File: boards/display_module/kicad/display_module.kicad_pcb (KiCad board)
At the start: 2 copper layers, 58.4 x 148.6 mm, 35 parts, among them IC1 ATMEGA328-P, P1 CONN_01X02, Q1 NDP6020P, Q2 NDP6020P, Q3 NDP6020P, Q4 NDP6020P, Q5 NDP6020P, Q6 NDP6020P, Q7 NDP6020P, Q8 NDP6020P, U1 TLC5940NT, U2 TLC5940NT, Y1 16M

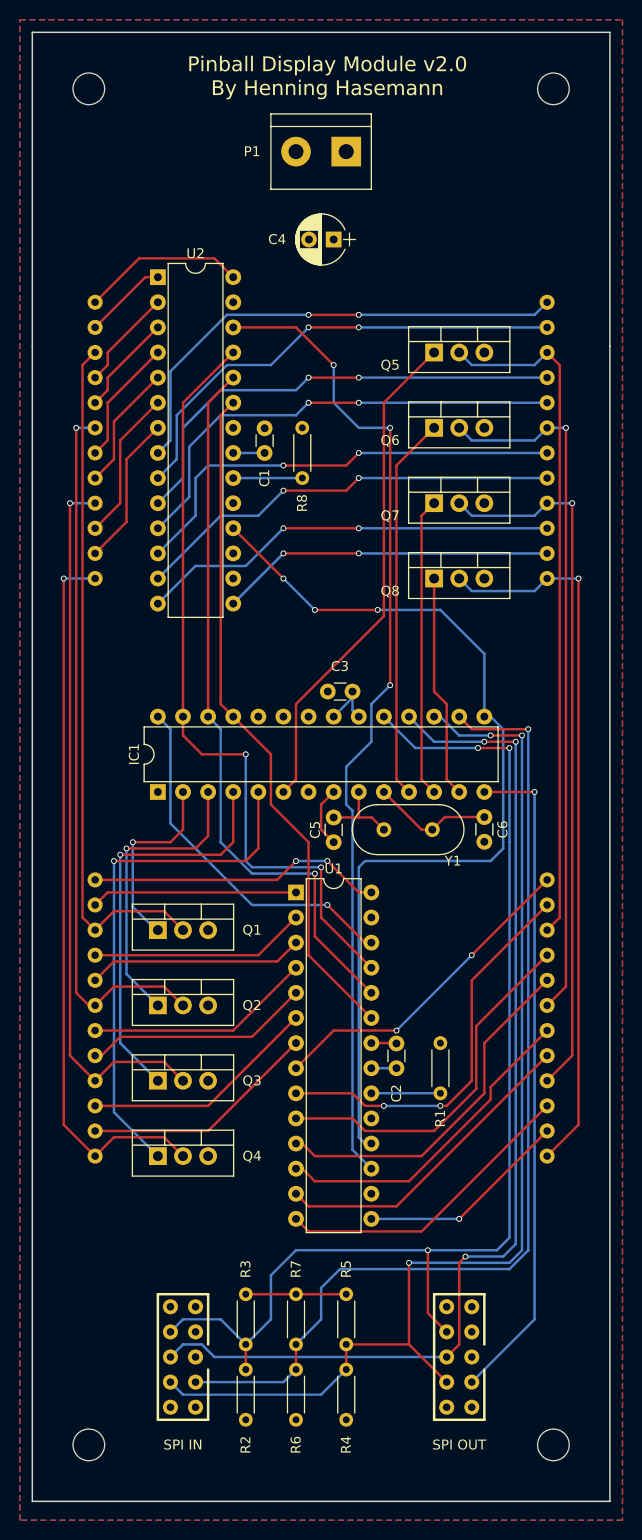
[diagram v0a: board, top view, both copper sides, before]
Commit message: WIP: display module PCB design v2.1
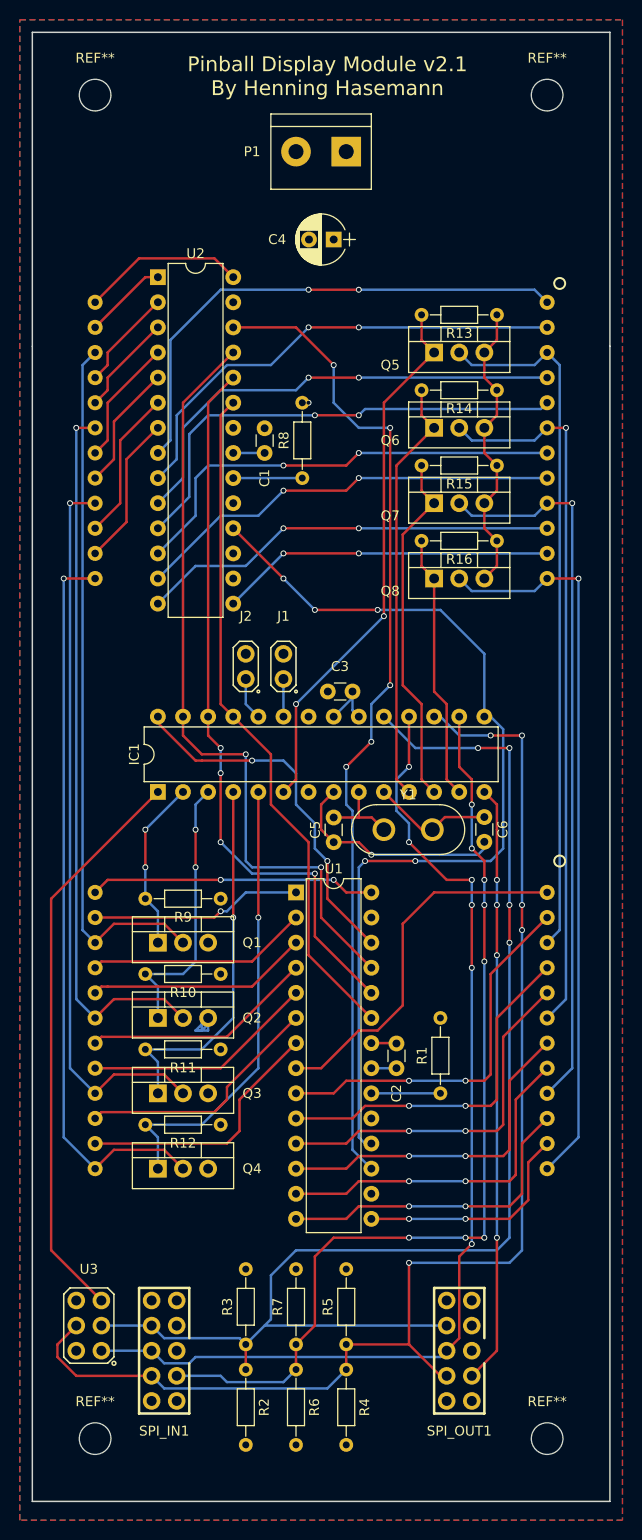
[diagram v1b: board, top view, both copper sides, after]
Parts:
- removed ? (x4): , Mounting_Holes:MountingHole_3.2mm_M3_DIN965
- removed SPI IN: SW10, my_footprints:SW10
- removed SPI OUT: SW10, my_footprints:SW10
- added J1: SELFTEST, my_footprints:PINS1x2, F.Cu at (144.8, 104.8)
- added J2: AUX, my_footprints:PINS1x2, F.Cu at (141.0, 104.8)
- added R10: 10k, Resistors_ThroughHole:R_Axial_DIN0204_L3.6mm_D1.6mm_P7.62mm_Horizontal, F.Cu at (138.4, 139.7)
- added R11: 10k, Resistors_ThroughHole:R_Axial_DIN0204_L3.6mm_D1.6mm_P7.62mm_Horizontal, F.Cu at (138.4, 147.3)
- added R12: 10k, Resistors_ThroughHole:R_Axial_DIN0204_L3.6mm_D1.6mm_P7.62mm_Horizontal, F.Cu at (138.4, 154.9)
- added R13: 10k, Resistors_ThroughHole:R_Axial_DIN0204_L3.6mm_D1.6mm_P7.62mm_Horizontal, F.Cu at (166.4, 73.0)
- added R14: 10k, Resistors_ThroughHole:R_Axial_DIN0204_L3.6mm_D1.6mm_P7.62mm_Horizontal, F.Cu at (166.4, 80.6)
- added R15: 10k, Resistors_ThroughHole:R_Axial_DIN0204_L3.6mm_D1.6mm_P7.62mm_Horizontal, F.Cu at (166.4, 88.3)
- added R16: 10k, Resistors_ThroughHole:R_Axial_DIN0204_L3.6mm_D1.6mm_P7.62mm_Horizontal, F.Cu at (166.4, 95.9)
- added R9: 10k, Resistors_ThroughHole:R_Axial_DIN0204_L3.6mm_D1.6mm_P7.62mm_Horizontal, F.Cu at (138.4, 132.1)
- added REF**: MountingHole_3.2mm_M3_ISO14580, Mounting_Holes:MountingHole_3.2mm_M3_ISO14580, F.Cu at (171.4, 50.8)
- added REF**: MountingHole_3.2mm_M3_ISO14580, Mounting_Holes:MountingHole_3.2mm_M3_ISO14580, F.Cu at (125.7, 50.8)
- added REF**: MountingHole_3.2mm_M3_ISO14580, Mounting_Holes:MountingHole_3.2mm_M3_ISO14580, F.Cu at (125.7, 186.7)
- added REF**: MountingHole_3.2mm_M3_ISO14580, Mounting_Holes:MountingHole_3.2mm_M3_ISO14580, F.Cu at (171.4, 186.7)
- added SPI_IN1: SW10, my_footprints:SW10, F.Cu at (132.7, 185.4)
- added SPI_OUT1: SW10, my_footprints:SW10, F.Cu at (162.6, 185.4)
- added U3: ICSP, my_footprints:PINS3x2, F.Cu at (125.1, 170.8)
- P1: value CONN_01X02 -> POWER
- R1, R2, R3, R4, R5, R6, R7, R8: footprint Resistors_ThroughHole:R_Axial_DIN0204_L3.6mm_D1.6mm_P5.08mm_Horizontal -> Resistors_ThroughHole:R_Axial_DIN0204_L3.6mm_D1.6mm_P7.62mm_Horizontal
- Y1: footprint Crystals:Crystal_HC18-U_Vertical -> Crystals:Crystal_HC50_Vertical
- moved Q1 1.27 mm to (132.1, 136.5)
- moved Q2 1.27 mm to (132.1, 144.1)
- moved DISP1 1.27 mm to (148.6, 141.6)
- moved Q3 1.27 mm to (132.1, 151.8)
- moved Q4 1.27 mm to (132.1, 159.4)
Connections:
- IC1 pad 1: (no net) -> Net-(IC1-Pad1)
- IC1 pad 23: (no net) -> Net-(IC1-Pad23)
- IC1 pad 24: (no net) -> Net-(IC1-Pad24)
- U1 pad 16: (no net) -> Net-(U1-Pad16)
- U2 pad 16: (no net) -> Net-(U2-Pad16)
- U2 pad 17: (no net) -> Net-(U2-Pad17)
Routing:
- net Net-(IC1-Pad1): track 0.00 -> 58.0 mm
- net VCC: track 22.0 -> 51.5 mm
- net GND: track 8.69 -> 25.4 mm, vias 0 -> 2
- net Net-(IC1-Pad17): track 115.6 -> 131.3 mm, vias 3 -> 5
- net Net-(IC1-Pad19): track 118.1 -> 133.6 mm, vias 3 -> 4
- net Net-(IC1-Pad14): track 67.4 -> 60.6 mm, vias 1 -> 4
- net Net-(IC1-Pad16): track 102.7 -> 96.8 mm, vias 1 -> 8
- net Net-(IC1-Pad12): track 30.3 -> 36.2 mm
- net Net-(IC1-Pad5): track 52.5 -> 46.7 mm
- net Net-(IC1-Pad11): track 38.9 -> 43.3 mm, vias 0 -> 1
- net Net-(IC1-Pad24): track 0.00 -> 4.34 mm
- net Net-(IC1-Pad13): track 22.6 -> 27.0 mm
- net Net-(IC1-Pad6): track 50.8 -> 55.1 mm, vias 0 -> 2
- net Net-(DISP1-Pad1): track 33.3 -> 37.6 mm, vias 2 -> 0
- net Net-(IC1-Pad23): track 0.00 -> 3.81 mm
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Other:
- board text added: "Pinball Display Module v2.1 By Henning Hasemann"
- board text removed: "Pinball Display Module v2.0 By Henning Hasemann"
